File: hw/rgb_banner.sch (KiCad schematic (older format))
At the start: 8 parts, among them P1 TST, P2 TST, P3 TST, P4 TST, U1 WS2812B, U2 WS2812B, U3 WS2812B, U4 WS2812B

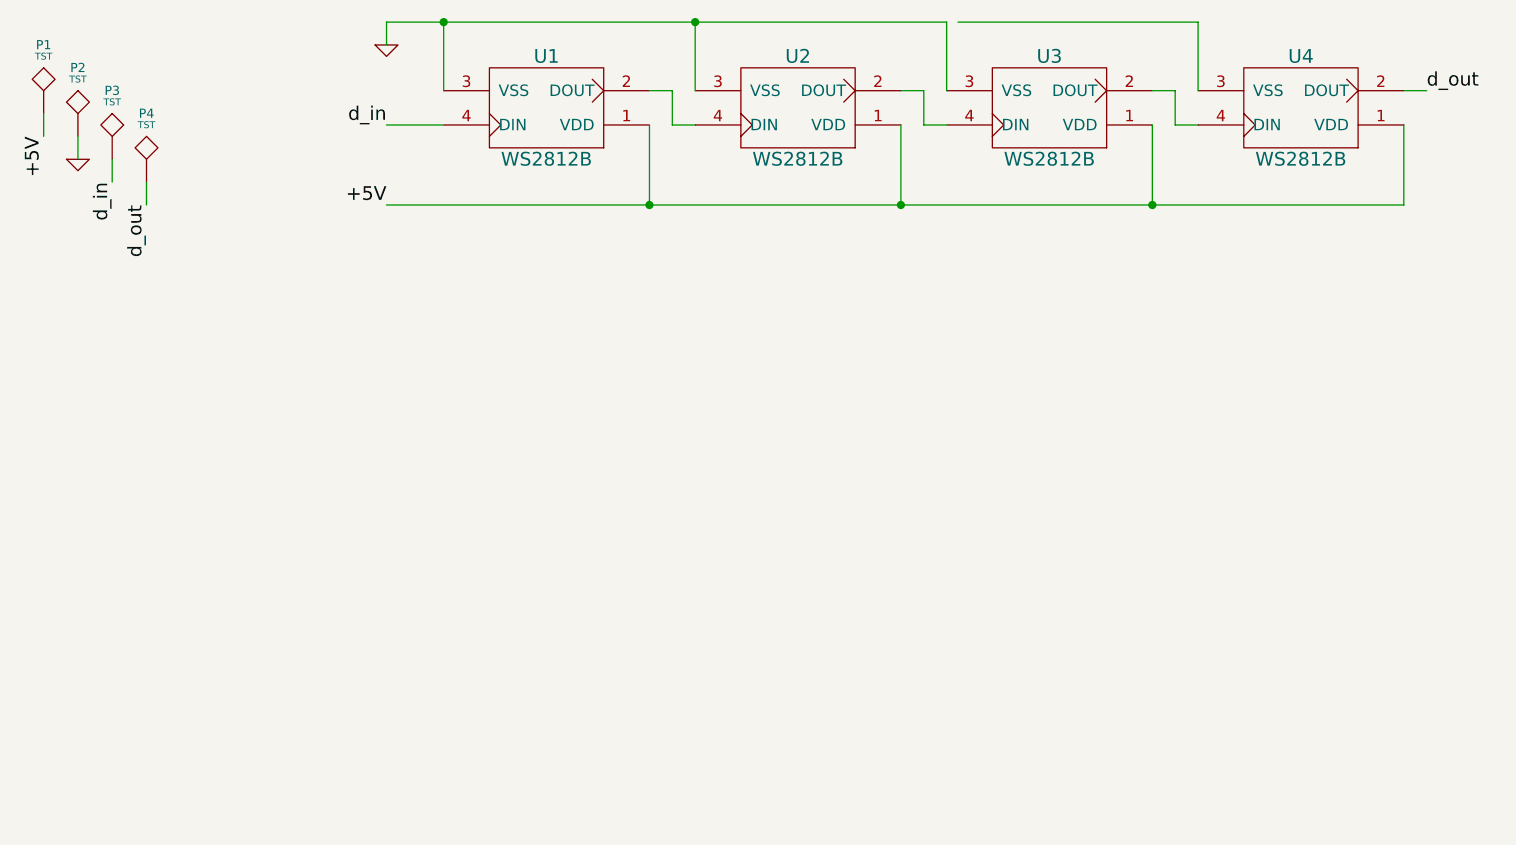
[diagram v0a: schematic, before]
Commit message: schematic pretty much done, start layout
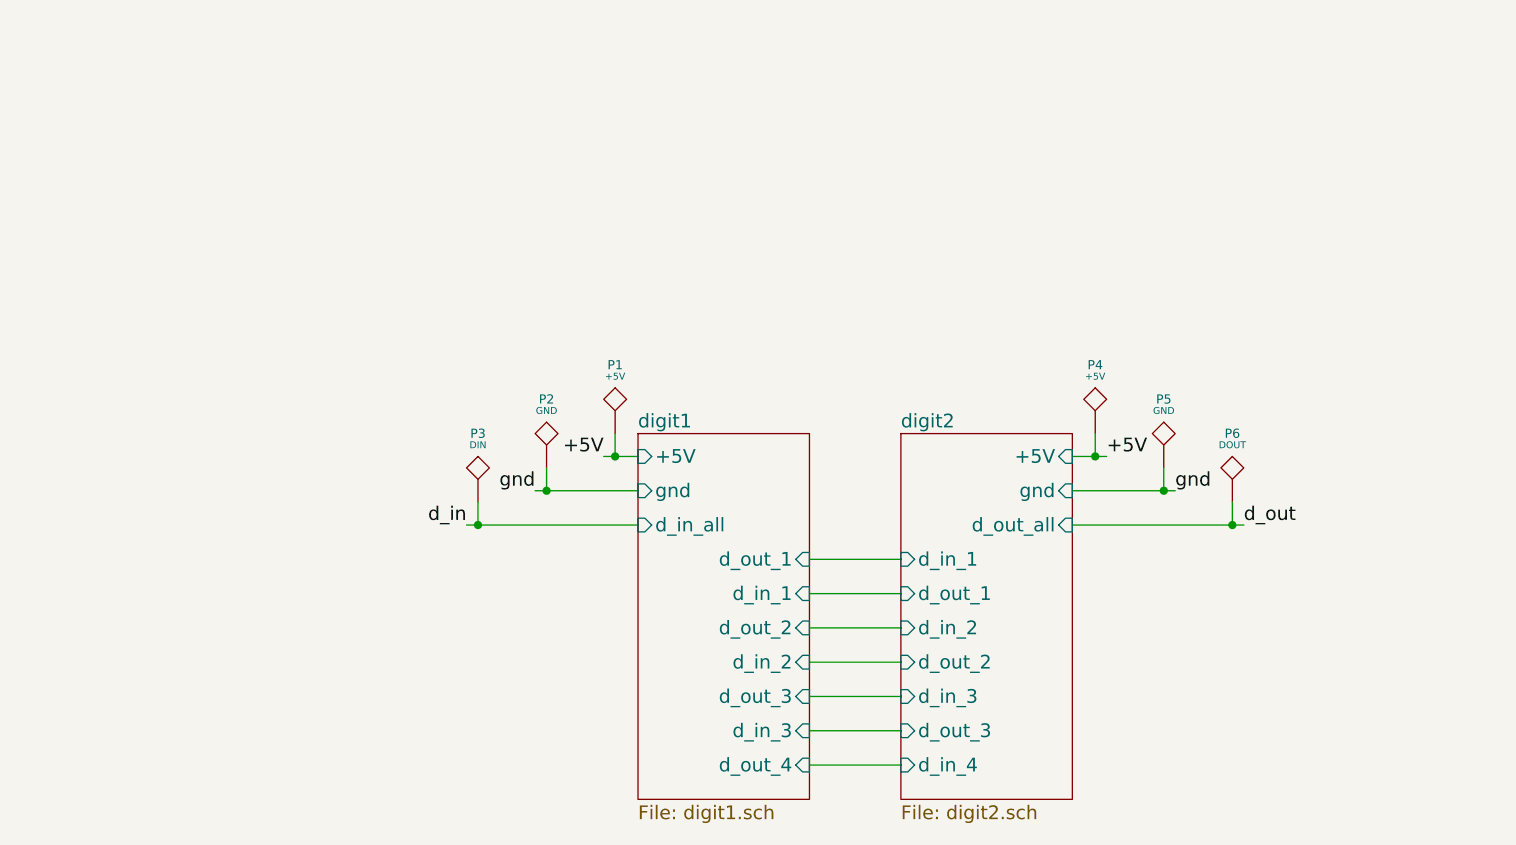
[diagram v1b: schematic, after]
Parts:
- removed U1, U2, U3, U4: WS2812B, symbol WS2812B
- added P4: +5V, kicadlib:TEST_0.100, symbol TST
- added P5: GND, kicadlib:TEST_0.100, symbol TST
- P1: value TST -> +5V; footprint (none) -> kicadlib:TEST_0.100
- P2: value TST -> GND; footprint (none) -> kicadlib:TEST_0.100
- P3: value TST -> DIN; footprint (none) -> kicadlib:TEST_0.100
- P6: renamed from P4; value TST -> DOUT; footprint (none) -> kicadlib:TEST_0.100
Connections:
- net labels added: gnd
- net labels removed: GND
- wire segments 27 -> 19
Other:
- moved on the sheet: P1, P2, P3, P6
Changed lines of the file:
@@
 $Descr A4 11693 8268
 encoding utf-8
-Sheet 1 1
+Sheet 1 3
 Title ""
 Date ""
@@
 $EndDescr
 $Comp
-L WS2812B U1
-U 1 1 556C6577
-P 4050 2100
-F 0 "U1" H 4050 1850 60  0000 C CNN
-F 1 "WS2812B" H 4050 2300 60  0000 C CNN
-F 2 "" H 4350 1950 60  0000 C CNN
-F 3 "" H 4350 1950 60  0000 C CNN
-	1    4050 2100
-	-1   0    0    1
-$EndComp
-$Comp
-L WS2812B U2
-U 1 1 556C661E
-P 5150 2100
-F 0 "U2" H 5150 1850 60  0000 C CNN
-F 1 "WS2812B" H 5150 2300 60  0000 C CNN
-F 2 "" H 5450 1950 60  0000 C CNN
-F 3 "" H 5450 1950 60  0000 C CNN
-	1    5150 2100
-	-1   0    0    1
-$EndComp
-$Comp
-L WS2812B U3
-U 1 1 556C6646
-P 6250 2100
-F 0 "U3" H 6250 1850 60  0000 C CNN
-F 1 "WS2812B" H 6250 2300 60  0000 C CNN
-F 2 "" H 6550 1950 60  0000 C CNN
-F 3 "" H 6550 1950 60  0000 C CNN
-	1    6250 2100
-	-1   0    0    1
-$EndComp
-$Comp
-L WS2812B U4
-U 1 1 556C6673
-P 7350 2100
-F 0 "U4" H 7350 1850 60  0000 C CNN
-F 1 "WS2812B" H 7350 2300 60  0000 C CNN
-F 2 "" H 7650 1950 60  0000 C CNN
-F 3 "" H 7650 1950 60  0000 C CNN
-	1    7350 2100
-	-1   0    0    1
-$EndComp
-Text Label 3350 2500 2    60   ~ 0
-+5V
-$Comp
-L GND #PWR01
-U 1 1 556C66A2
-P 3350 1800
-F 0 "#PWR01" H 3350 1800 30  0001 C CNN
-F 1 "GND" H 3350 1730 30  0001 C CNN
-F 2 "" H 3350 1800 60  0000 C CNN
-F 3 "" H 3350 1800 60  0000 C CNN
-	1    3350 1800
-	1    0    0    -1
-$EndComp
-Wire Wire Line
-	3600 2000 3600 1700
-Wire Wire Line
-	3350 1700 5800 1700
-Wire Wire Line
-	3350 1700 3350 1800
-Text Label 3350 2150 2    60   ~ 0
-d_in
-Wire Wire Line
-	3350 2150 3600 2150
-Wire Wire Line
-	3350 2500 7800 2500
-Wire Wire Line
-	4500 2500 4500 2150
-Wire Wire Line
-	4500 2000 4600 2000
-Wire Wire Line
-	4600 2000 4600 2150
-Wire Wire Line
-	4600 2150 4700 2150
-Wire Wire Line
-	5600 2000 5700 2000
-Wire Wire Line
-	5700 2000 5700 2150
-Wire Wire Line
-	5700 2150 5800 2150
-Wire Wire Line
-	5600 2500 5600 2150
-Connection ~ 4500 2500
-Wire Wire Line
-	4700 1700 4700 2000
-Connection ~ 3600 1700
-Wire Wire Line
-	5800 1700 5800 2000
-Connection ~ 4700 1700
-Wire Wire Line
-	5850 1700 6900 1700
-Wire Wire Line
-	6900 1700 6900 2000
-Wire Wire Line
-	6700 2500 6700 2150
-Connection ~ 5600 2500
-Wire Wire Line
-	7800 2500 7800 2150
-Connection ~ 6700 2500
-Wire Wire Line
-	6700 2000 6800 2000
-Wire Wire Line
-	6800 2000 6800 2150
-Wire Wire Line
-	6800 2150 6900 2150
-Text Label 7900 2000 0    60   ~ 0
-d_out
-Wire Wire Line
-	7900 2000 7800 2000
-$Comp
 L TST P1
 U 1 1 556C686B
-P 1850 2100
-F 0 "P1" H 1850 2400 40  0000 C CNN
-F 1 "TST" H 1850 2350 30  0000 C CNN
-F 2 "" H 1850 2100 60  0000 C CNN
-F 3 "" H 1850 2100 60  0000 C CNN
-	1    1850 2100
+P 4350 3500
+F 0 "P1" H 4350 3800 40  0000 C CNN
+F 1 "+5V" H 4350 3750 30  0000 C CNN
+F 2 "kicadlib:TEST_0.100" H 4350 3500 60  0001 C CNN
+F 3 "" H 4350 3500 60  0000 C CNN
+	1    4350 3500
 	1    0    0    -1
 $EndComp
@@
 L TST P2
 U 1 1 556C69BB
-P 2000 2200
-F 0 "P2" H 2000 2500 40  0000 C CNN
-F 1 "TST" H 2000 2450 30  0000 C CNN
-F 2 "" H 2000 2200 60  0000 C CNN
-F 3 "" H 2000 2200 60  0000 C CNN
-	1    2000 2200
+P 4050 3650
+F 0 "P2" H 4050 3950 40  0000 C CNN
+F 1 "GND" H 4050 3900 30  0000 C CNN
+F 2 "kicadlib:TEST_0.100" H 4050 3650 60  0001 C CNN
+F 3 "" H 4050 3650 60  0000 C CNN
+	1    4050 3650
 	1    0    0    -1
 $EndComp
@@
 L TST P3
 U 1 1 556C69DB
-P 2150 2300
-F 0 "P3" H 2150 2600 40  0000 C CNN
-F 1 "TST" H 2150 2550 30  0000 C CNN
-F 2 "" H 2150 2300 60  0000 C CNN
-F 3 "" H 2150 2300 60  0000 C CNN
-	1    2150 2300
+P 3750 3800
+F 0 "P3" H 3750 4100 40  0000 C CNN
+F 1 "DIN" H 3750 4050 30  0000 C CNN
+F 2 "kicadlib:TEST_0.100" H 3750 3800 60  0001 C CNN
+F 3 "" H 3750 3800 60  0000 C CNN
+	1    3750 3800
 	1    0    0    -1
 $EndComp
 $Comp
-L TST P4
+L TST P6
 U 1 1 556C69FA
-P 2300 2400
-F 0 "P4" H 2300 2700 40  0000 C CNN
-F 1 "TST" H 2300 2650 30  0000 C CNN
-F 2 "" H 2300 2400 60  0000 C CNN
-F 3 "" H 2300 2400 60  0000 C CNN
-	1    2300 2400
+P 7050 3800
+F 0 "P6" H 7050 4100 40  0000 C CNN
+F 1 "DOUT" H 7050 4050 30  0000 C CNN
+F 2 "kicadlib:TEST_0.100" H 7050 3800 60  0001 C CNN
+F 3 "" H 7050 3800 60  0000 C CNN
+	1    7050 3800
 	1    0    0    -1
 $EndComp
-Text Label 1850 2200 3    60   ~ 0
+Text Label 4300 3600 2    60   ~ 0
 +5V
+Text Label 3700 3900 2    60   ~ 0
+d_in
+Text Label 7100 3900 0    60   ~ 0
+d_out
+Wire Wire Line
+	3750 3800 3750 3900
+Wire Wire Line
+	4050 3750 4050 3650
+Wire Wire Line
+	4350 3600 4350 3500
 $Comp
-L GND #PWR02
-U 1 1 556C6A24
-P 2000 2300
-F 0 "#PWR02" H 2000 2300 30  0001 C CNN
-F 1 "GND" H 2000 2230 30  0001 C CNN
-F 2 "" H 2000 2300 60  0000 C CNN
-F 3 "" H 2000 2300 60  0000 C CNN
-	1    2000 2300
+L TST P4
+U 1 1 556C71D9
+P 6450 3500
+F 0 "P4" H 6450 3800 40  0000 C CNN
+F 1 "+5V" H 6450 3750 30  0000 C CNN
+F 2 "kicadlib:TEST_0.100" H 6450 3500 60  0001 C CNN
+F 3 "" H 6450 3500 60  0000 C CNN
+	1    6450 3500
 	1    0    0    -1
 $EndComp
-Text Label 2150 2400 3    60   ~ 0
-d_in
-Text Label 2300 2500 3    60   ~ 0
-d_out
+$Comp
+L TST P5
+U 1 1 556C71DF
+P 6750 3650
+F 0 "P5" H 6750 3950 40  0000 C CNN
+F 1 "GND" H 6750 3900 30  0000 C CNN
+F 2 "kicadlib:TEST_0.100" H 6750 3650 60  0001 C CNN
+F 3 "" H 6750 3650 60  0000 C CNN
+	1    6750 3650
+	1    0    0    -1
+$EndComp
+Text Label 6500 3600 0    60   ~ 0
++5V
 Wire Wire Line
-	2300 2500 2300 2400
+	6450 3600 6450 3500
+Text Label 4000 3750 2    60   ~ 0
+gnd
+$Sheet
+S 5600 3500 750  1600
+U 556C8A1A
+F0 "digit2" 60
+F1 "digit2.sch" 60
+F2 "gnd" I R 6350 3750 60
+F3 "+5V" I R 6350 3600 60
+F4 "d_in_1" I L 5600 4050 60
+F5 "d_out_all" I R 6350 3900 60
+F6 "d_in_2" I L 5600 4350 60
+F7 "d_in_3" I L 5600 4650 60
+F8 "d_out_1" I L 5600 4200 60
+F9 "d_out_2" I L 5600 4500 60
+F10 "d_out_3" I L 5600 4800 60
+F11 "d_in_4" I L 5600 4950 60
+$EndSheet
 Wire Wire Line
-	2150 2300 2150 2400
+	3700 3900 4450 3900
 Wire Wire Line
-	2000 2300 2000 2200
+	4000 3750 4450 3750
 Wire Wire Line
-	1850 2200 1850 2100
+	4300 3600 4450 3600
+Connection ~ 4350 3600
+Connection ~ 4050 3750
+Connection ~ 3750 3900
+Text Label 6800 3750 0    60   ~ 0
+gnd
+Wire Wire Line
+	6350 3600 6500 3600
+Connection ~ 6450 3600
+Wire Wire Line
+	6350 3750 6800 3750
+Wire Wire Line
+	6750 3750 6750 3650
+Wire Wire Line
+	6350 3900 7100 3900
+Wire Wire Line
+	7050 3900 7050 3800
+Connection ~ 6750 3750
+Connection ~ 7050 3900
+$Sheet
+S 4450 3500 750  1600
+U 556C8146
+F0 "digit1" 60
+F1 "digit1.sch" 60
+F2 "gnd" I L 4450 3750 60
+F3 "+5V" I L 4450 3600 60
+F4 "d_in_all" I L 4450 3900 60
+F5 "d_out_3" I R 5200 4650 60
+F6 "d_out_4" I R 5200 4950 60
+F7 "d_in_3" I R 5200 4800 60
+F8 "d_in_2" I R 5200 4500 60
+F9 "d_out_2" I R 5200 4350 60
+F10 "d_in_1" I R 5200 4200 60
+F11 "d_out_1" I R 5200 4050 60
+$EndSheet
+Wire Wire Line
+	5200 4050 5600 4050
+Wire Wire Line
+	5600 4200 5200 4200
+Wire Wire Line
+	5200 4350 5600 4350
+Wire Wire Line
+	5600 4500 5200 4500
+Wire Wire Line
+	5200 4650 5600 4650
+Wire Wire Line
+	5600 4800 5200 4800
+Wire Wire Line
+	5200 4950 5600 4950
 $EndSCHEMATC
